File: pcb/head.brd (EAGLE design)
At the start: 41.6 x 21.6 mm, 9 parts

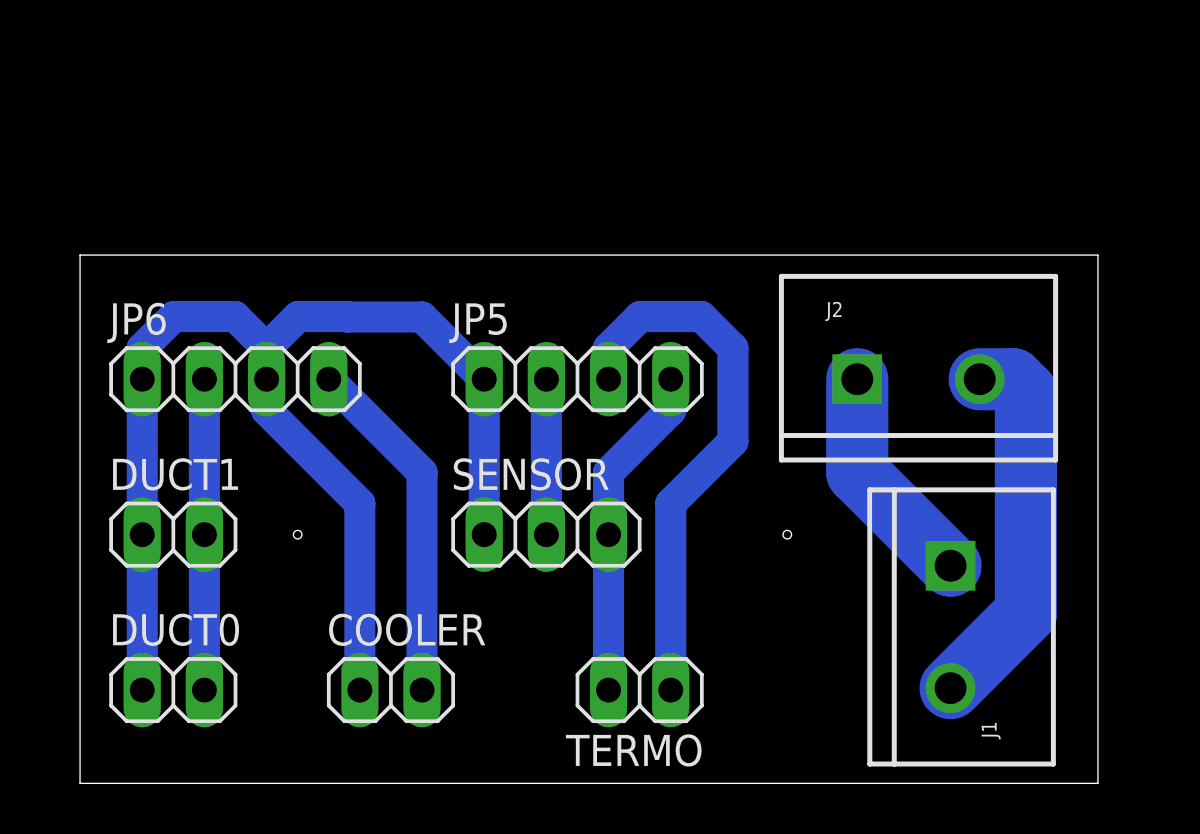
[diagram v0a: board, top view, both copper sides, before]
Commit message: pcb
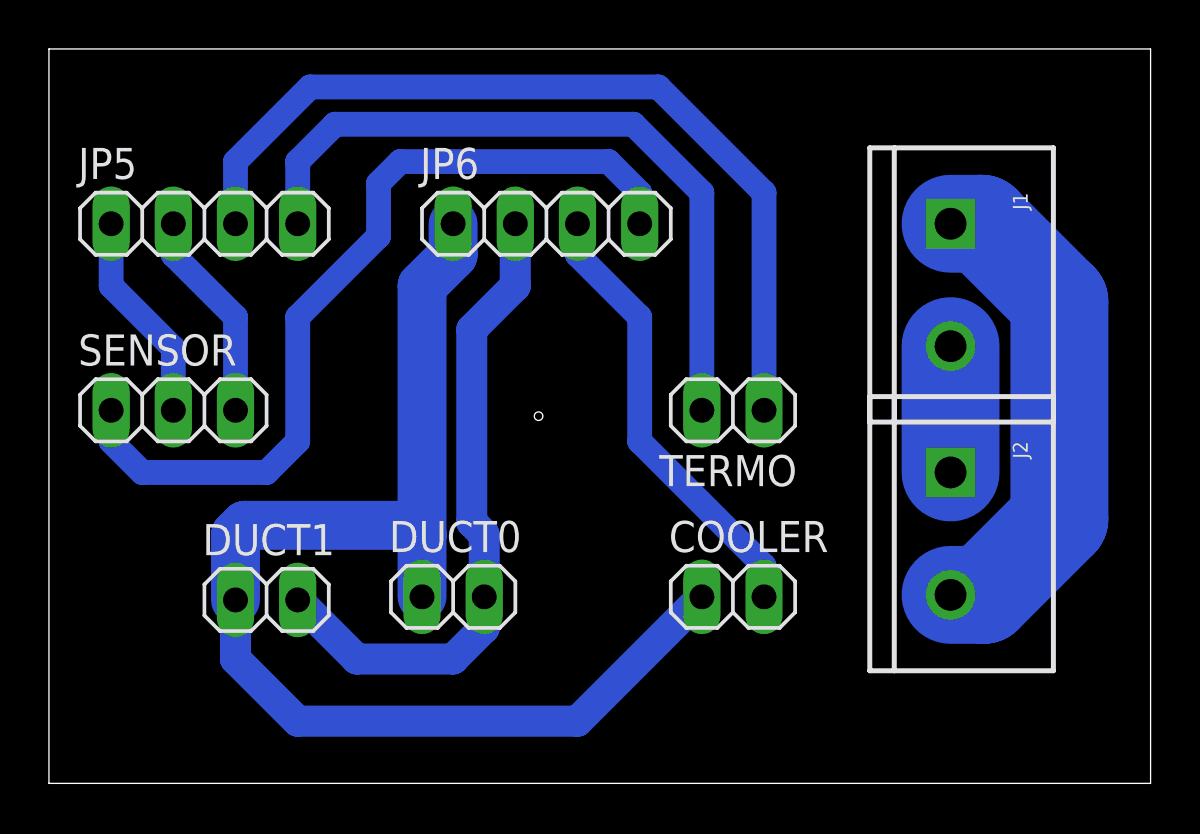
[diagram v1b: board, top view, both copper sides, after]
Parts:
- moved JP5 16.5 mm to (6.35, 22.9)
- moved SENSOR 16.1 mm to (5.08, 15.2)
- moved COOLER 14.5 mm to (27.9, 7.62)
- moved JP6 14.2 mm to (20.3, 22.9)
- moved J1 14.0 mm to (36.8, 22.9)
- moved DUCT0 12.0 mm to (16.5, 7.62)
- moved TERMO 12.0 mm to (27.9, 15.2)
- moved J2 5.39 mm to (36.8, 12.7), turned to 270 degrees
- moved DUCT1 4.65 mm to (8.89, 7.49)
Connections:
- new net 5V: JP6.4, SENSOR.1
- new net N$4: J1.1, J2.2
- net GND: now also JP5.2; no longer JP5.4, TERMO.2
- net N$1: now also JP5.1, SENSOR.2; no longer J1.1, J2.1
- net N$2: now also COOLER.2, JP6.3; no longer J1.2, J2.2
- net N$5: now also JP5.4, TERMO.2; no longer COOLER.2, JP6.4
- net N$6: now also J1.2, J2.1; no longer JP5.2, SENSOR.2
- net VCC: no longer JP5.1, JP6.3, SENSOR.1
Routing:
- net 5V: track 0.00 -> 34.7 mm
- net N$4: track 0.00 -> 20.4 mm
- net N$5: track 14.3 -> 29.7 mm
- net N$9: track 12.7 -> 26.6 mm
- net N$3: track 22.4 -> 36.1 mm
- net GND: track 13.8 -> 8.67 mm
- net N$2: track 15.5 -> 18.4 mm
- net VCC: track 52.5 -> 51.0 mm
- net N$6: track 6.35 -> 5.16 mm
- net N$1: track 9.20 -> 8.67 mm
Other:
- board size 41.6 x 21.6 mm -> 45 x 30 mm
